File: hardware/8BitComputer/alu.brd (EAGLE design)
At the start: 100 x 75 mm, 32 parts, among them IC1 SN74LS245NE4, IC2 SN74LS86AN, IC3 SN74LS283N, IC4 SN74LS86AN, IC8 SN74LS283N

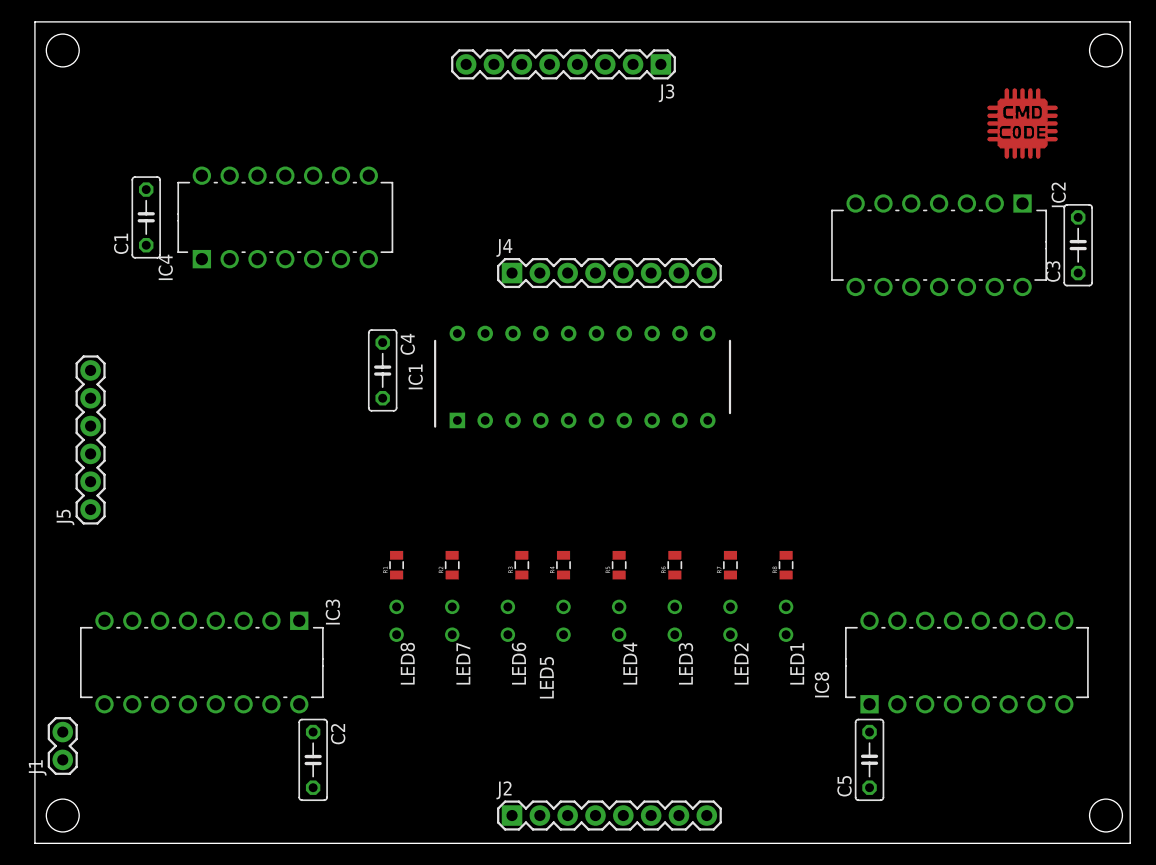
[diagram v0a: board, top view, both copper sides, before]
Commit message: alu routed
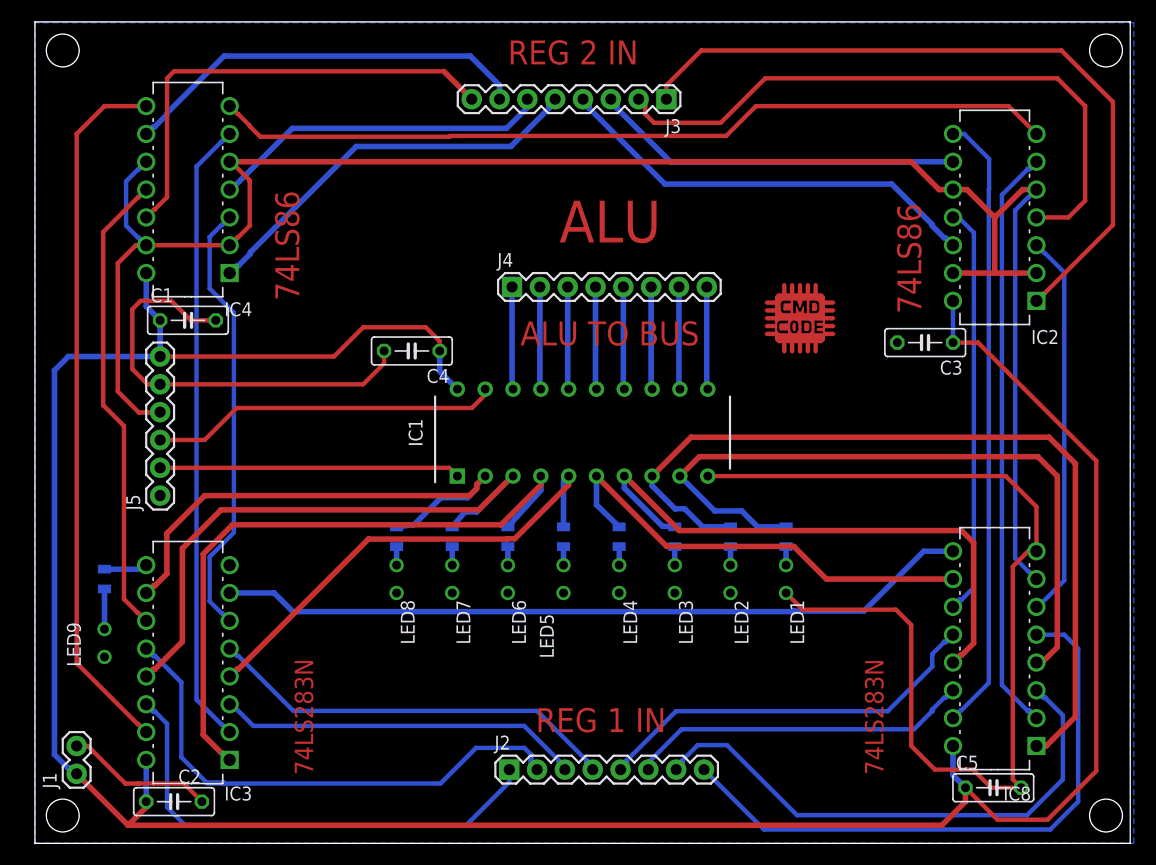
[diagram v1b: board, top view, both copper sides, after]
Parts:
- added LED9: RED, leds:LED3MM-NS
- added R9: 100 R, passives:0805
- moved U$1 27.0 mm to (69.8, 48.3)
- moved IC4 21.3 mm to (10.2, 67.3), turned to 180 degrees
- moved C3 16.6 mm to (81.3, 45.7), turned to 180 degrees
- moved IC2 16.6 mm to (83.8, 64.8), turned to 180 degrees
- moved C2 13.3 mm to (12.7, 3.81), turned to 0 degrees
- moved IC3 13.3 mm to (10.2, 25.4), turned to 180 degrees
- moved IC8 12.0 mm to (83.8, 26.7), turned to 180 degrees
- moved C5 11.6 mm to (87.5, 5.08), turned to 0 degrees
- moved C1 10.1 mm to (14.0, 47.8), turned to 0 degrees
- moved J5 6.48 mm to (11.4, 31.8)
- moved IC1 5.08 mm to (50.0, 37.5)
- moved J2 4.20 mm to (43.3, 6.73)
- moved LED1 3.81 mm to (68.6, 24.1)
- moved LED2 3.81 mm to (63.5, 24.1)
- moved LED3 3.81 mm to (58.4, 24.1)
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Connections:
- removed net N$6: J5.5
- new net N$10: IC3.9, R9.1
- new net N$11: LED9.A, R9.2
- net ALUOUT_OE: now also J5.3; no longer J5.2
- net AO_DIR: now also J5.2; no longer J5.3
- net AR2O_2: now also IC8.15
- net AR2O_3: no longer IC8.15
- net CARRY_ADD: now also IC3.7, IC8.9; no longer IC3.9, IC8.7
- net GND: now also J5.5, LED9.K
- net OP_SUBTRACT: now also IC8.7; no longer IC8.9
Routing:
- net VCC5V: track 0.00 -> 249.2 mm
- net GND: track 0.00 -> 224.0 mm
- net OP_SUBTRACT: track 0.00 -> 172.5 mm
- net AO_1: track 0.00 -> 78.5 mm
- net CARRY_ADD: track 0.00 -> 69.0 mm
- net AR2_0: track 0.00 -> 66.4 mm
- net AO_0: track 0.00 -> 65.6 mm
- net AR2O_6: track 0.00 -> 64.7 mm
- net AO_5: track 0.00 -> 59.9 mm
- net AR2_1: track 0.00 -> 58.5 mm
- net AR2O_5: track 0.00 -> 57.2 mm
- net AR2O_2: track 0.00 -> 56.7 mm
- net AR1_BUS0: track 0.00 -> 55.8 mm
- net AO_6: track 0.00 -> 53.6 mm
- net AR2O_1: track 0.00 -> 53.6 mm
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- added copper zone on layer 16, net GND
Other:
- board text added: "74LS283N"
- board text added: "74LS86"
- board text added: "ALU"
- board text added: "ALU TO BUS"
- board text added: "REG 1 IN"
- board text added: "REG 2 IN"
